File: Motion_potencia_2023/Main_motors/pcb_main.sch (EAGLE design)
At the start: 22 parts, among them IC1 TEENSY_4.1, X5 5566-25569-2, X6 5566-25569-2, X7 5566-25569-2, X8 5566-25569-2

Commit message: main lista, sin revisión
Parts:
- removed 12V_VENT, 3.3_MD, 5V_TEENSY, MOUT5, MOUT6, MOUT7, MOUT8, X5, X6, X7, X8: 5566-25569-2, molex_arreglado_2:5566-25569-2
- added 12V_IN, VENT1, VENT2: (no value), pinhead:PINHD-1X2
- added 5_MD: 5566-25569-2, molex_arreglado_2:5566-25569-2
- added FUSEMD1, FUSEMD2: FUSEBLANK_5X20MM, fuse:FUSEBLANK_5X20MM
- added JP1, JP3, JP4: (no value), pinhead:PINHD-1X4
- added RGB1, RGB2: (no value), pinhead:PINHD-1X3
- added U$1, U$2, U$3, U$4: GX16_2_PINS, Robocol_Eagle_Libraries2:GX16_2_PINS
- JP2: device jumper:JP4Q -> pinhead:PINHD-1X4
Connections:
- removed net 3.3V: JP2.7
- removed net 3.3V_MD: 3.3_MD-2.S, MD_1.VIN, MD_2.VIN
- removed net 5V_TEENSY: 5V_TEENSY-2.S, IC1.VIN_(3.6_TO_5.5_VOLTS)
- removed net N$1: X7-2.S, X8-2.S
- removed net SCL_1: JP2.1
- removed net SCL_2: JP2.3
- removed net SDA_1: JP2.2
- removed net SDA_2: JP2.4
- new net 5V_MD: 5_MD-2.S, JP1.1, JP2.1, JP3.1, JP4.1, MD_1.VIN, MD_2.VIN, RGB1.1, RGB2.1
- new net A14: IC1.A14, JP4.2
- new net A15: IC1.A15, JP3.2
- new net A16: IC1.A16, JP2.2
- new net A17: IC1.A17, JP1.2
- new net D18: IC1.A4, JP2.4
- new net D19: IC1.A5, JP1.4
- new net D28: IC1.RX7, RGB1.2
- new net D29: IC1.TX7, RGB2.2
- new net D36: IC1.CS_2, JP4.4
- new net D37: IC1.CS_3, JP3.4
- new net FUSE20AMD1: 24V_IZQ-2.S, FUSEMD1.2
- new net FUSE20AMD2: 24V_DER-2.S, FUSEMD2.2
- net 12V_VENT: now also 12V_IN.2, VENT1.2, VENT2.2; no longer 12V_VENT-2.S, X5-2.S, X6-2.S
- net 24V_IN_MD: now also FUSEMD1.1, FUSEMD2.1; no longer 24V_DER-2.S, 24V_IZQ-2.S
- net GND: now also 12V_IN.1, 5_MD-1.S, JP1.3, JP2.3, JP3.3, JP4.3, RGB1.3, RGB2.3, VENT1.1, VENT2.1; no longer 12V_VENT-1.S, 3.3_MD-1.S, 5V_TEENSY-1.S, JP2.8, X5-1.S, X6-1.S, X7-1.S, X8-1.S
- net N$10: now also MOUT3-2.S, U$3.1; no longer MOUT4-2.S, MOUT8-2.S
- net N$3: now also U$1.3; no longer MOUT5-1.S
- net N$4: now also MOUT2-1.S, U$2.3; no longer MOUT1-2.S, MOUT5-2.S
- net N$5: now also MOUT2-2.S, U$2.1; no longer MOUT2-1.S, MOUT6-1.S
- net N$6: now also MOUT1-2.S, U$1.1; no longer MOUT2-2.S, MOUT6-2.S
- net N$7: now also MOUT4-1.S, U$4.3; no longer MOUT3-1.S, MOUT7-1.S
- net N$8: now also MOUT4-2.S, U$4.1; no longer MOUT3-2.S, MOUT7-2.S
- net N$9: now also MOUT3-1.S, U$3.3; no longer MOUT4-1.S, MOUT8-1.S
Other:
- moved on the sheet: 24V_DER-1, 24V_DER-2, 24V_IZQ-1, 24V_IZQ-2, IC1, MD_1, MD_2, MOUT1-1, MOUT1-2, MOUT2-1, MOUT2-2, MOUT3-1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

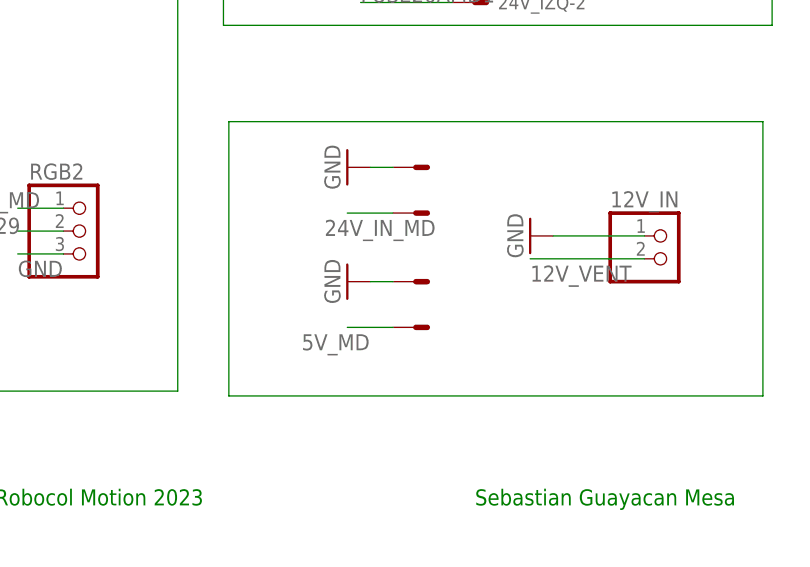
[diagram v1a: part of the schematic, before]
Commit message: main, power
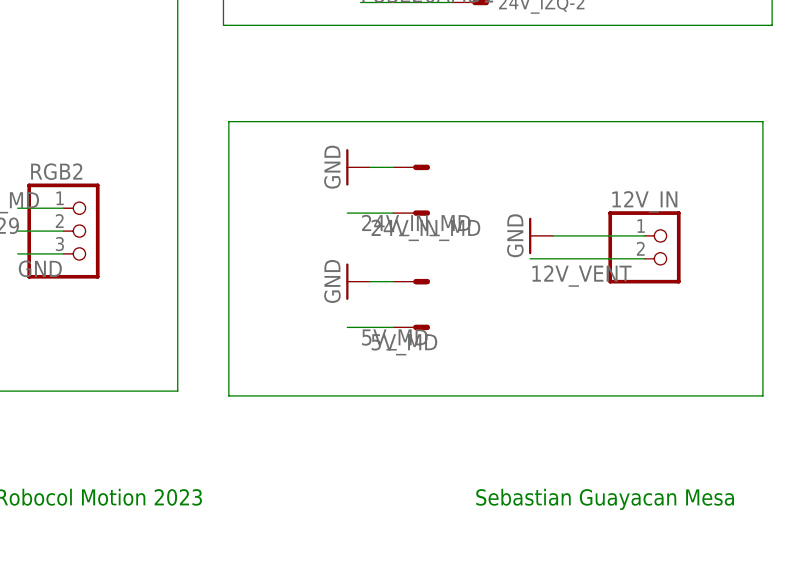
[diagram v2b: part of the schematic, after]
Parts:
- renumbered U$1 to M1, U$2 to M2, U$3 to M3, U$4 to M4
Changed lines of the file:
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@@
 <setting verticaltext="up"/>
 </settings>
-<grid distance="1" unitdist="mil" unit="mil" style="lines" multiple="1" display="no" altdistance="0.01" altunitdist="inch" altunit="inch"/>
+<grid distance="0.1" unitdist="inch" unit="inch" style="lines" multiple="1" display="no" altdistance="0.01" altunitdist="inch" altunit="inch"/>
 <layers>
 <layer number="1" name="Top" color="4" fill="1" visible="no" active="no"/>
@@
 <part name="GND5" library="supply1" library_urn="urn:adsk.eagle:library:371" deviceset="GND" device=""/>
 <part name="12V_IN" library="pinhead" library_urn="urn:adsk.eagle:library:325" deviceset="PINHD-1X2" device="" package3d_urn="urn:adsk.eagle:package:22435/2"/>
-<part name="U$1" library="Robocol_Eagle_Libraries2" deviceset="GX16_2_PINS" device=""/>
-<part name="U$2" library="Robocol_Eagle_Libraries2" deviceset="GX16_2_PINS" device=""/>
-<part name="U$3" library="Robocol_Eagle_Libraries2" deviceset="GX16_2_PINS" device=""/>
-<part name="U$4" library="Robocol_Eagle_Libraries2" deviceset="GX16_2_PINS" device=""/>
+<part name="M1" library="Robocol_Eagle_Libraries2" deviceset="GX16_2_PINS" device=""/>
+<part name="M2" library="Robocol_Eagle_Libraries2" deviceset="GX16_2_PINS" device=""/>
+<part name="M3" library="Robocol_Eagle_Libraries2" deviceset="GX16_2_PINS" device=""/>
+<part name="M4" library="Robocol_Eagle_Libraries2" deviceset="GX16_2_PINS" device=""/>
 <part name="FUSEMD1" library="fuse" library_urn="urn:adsk.eagle:library:233" deviceset="FUSE" device="BLANK_5X20MM" package3d_urn="urn:adsk.eagle:package:14079/1"/>
 <part name="FUSEMD2" library="fuse" library_urn="urn:adsk.eagle:library:233" deviceset="FUSE" device="BLANK_5X20MM" package3d_urn="urn:adsk.eagle:package:14079/1"/>
@@
 <attribute name="VALUE" x="233.47" y="42.64" size="1.778" layer="96"/>
 </instance>
-<instance part="U$1" gate="G$1" x="209.55" y="102.87" smashed="yes" rot="MR0"/>
-<instance part="U$2" gate="G$1" x="237.49" y="102.87" smashed="yes" rot="MR0"/>
-<instance part="U$3" gate="G$1" x="209.55" y="160.02" smashed="yes" rot="MR0"/>
-<instance part="U$4" gate="G$1" x="237.49" y="160.02" smashed="yes" rot="MR0"/>
+<instance part="M1" gate="G$1" x="209.55" y="102.87" smashed="yes" rot="MR0"/>
+<instance part="M2" gate="G$1" x="237.49" y="102.87" smashed="yes" rot="MR0"/>
+<instance part="M3" gate="G$1" x="209.55" y="160.02" smashed="yes" rot="MR0"/>
+<instance part="M4" gate="G$1" x="237.49" y="160.02" smashed="yes" rot="MR0"/>
 <instance part="FUSEMD1" gate="G$1" x="67.7418" y="19.1516" smashed="yes">
 <attribute name="NAME" x="63.9318" y="20.5486" size="1.778" layer="95"/>
@@
 <pinref part="24V_MD" gate="-2" pin="S"/>
 <wire x1="204.26" y1="52.8" x2="209.34" y2="52.8" width="0.1524" layer="91"/>
-<label x="201.72" y="50.26" size="1.778" layer="95"/>
+<label x="206.8" y="50.26" size="1.778" layer="95"/>
+<label x="205.74" y="50.8" size="1.778" layer="95"/>
 </segment>
 <segment>
@@
 <pinref part="5_MD" gate="-2" pin="S"/>
 <wire x1="209.34" y1="40.1" x2="204.26" y2="40.1" width="0.1524" layer="91"/>
-<label x="199.18" y="37.56" size="1.778" layer="95"/>
+<label x="206.8" y="37.56" size="1.778" layer="95"/>
+<label x="205.74" y="38.1" size="1.778" layer="95"/>
 </segment>
 <segment>
@@
 <net name="N$3" class="0">
 <segment>
-<pinref part="U$1" gate="G$1" pin="3"/>
+<pinref part="M1" gate="G$1" pin="3"/>
 <wire x1="198.12" y1="99.06" x2="198.12" y2="91.44" width="0.1524" layer="91"/>
 <pinref part="MOUT1" gate="-1" pin="S"/>
@@
 <segment>
 <pinref part="MOUT2" gate="-1" pin="S"/>
-<pinref part="U$2" gate="G$1" pin="3"/>
+<pinref part="M2" gate="G$1" pin="3"/>
 <wire x1="231.14" y1="91.44" x2="226.06" y2="91.44" width="0.1524" layer="91"/>
 <wire x1="226.06" y1="91.44" x2="226.06" y2="99.06" width="0.1524" layer="91"/>
@@
 <net name="N$5" class="0">
 <segment>
-<pinref part="U$2" gate="G$1" pin="1"/>
+<pinref part="M2" gate="G$1" pin="1"/>
 <wire x1="226.06" y1="106.68" x2="224.79" y2="106.68" width="0.1524" layer="91"/>
 <wire x1="224.79" y1="106.68" x2="224.79" y2="86.36" width="0.1524" layer="91"/>
@@
 <net name="N$6" class="0">
 <segment>
-<pinref part="U$1" gate="G$1" pin="1"/>
+<pinref part="M1" gate="G$1" pin="1"/>
 <wire x1="198.12" y1="106.68" x2="196.85" y2="105.41" width="0.1524" layer="91"/>
 <pinref part="MOUT1" gate="-2" pin="S"/>
@@
 <pinref part="MOUT4" gate="-1" pin="S"/>
 <wire x1="231.14" y1="149.86" x2="226.06" y2="149.86" width="0.1524" layer="91"/>
-<pinref part="U$4" gate="G$1" pin="3"/>
+<pinref part="M4" gate="G$1" pin="3"/>
 <wire x1="226.06" y1="149.86" x2="226.06" y2="156.21" width="0.1524" layer="91"/>
 </segment>
@@
 <wire x1="231.14" y1="144.78" x2="224.79" y2="144.78" width="0.1524" layer="91"/>
 <wire x1="224.79" y1="144.78" x2="224.79" y2="163.83" width="0.1524" layer="91"/>
-<pinref part="U$4" gate="G$1" pin="1"/>
+<pinref part="M4" gate="G$1" pin="1"/>
 <wire x1="224.79" y1="163.83" x2="226.06" y2="163.83" width="0.1524" layer="91"/>
 </segment>
@@
 <pinref part="MOUT3" gate="-1" pin="S"/>
 <wire x1="203.2" y1="148.59" x2="198.12" y2="148.59" width="0.1524" layer="91"/>
-<pinref part="U$3" gate="G$1" pin="3"/>
+<pinref part="M3" gate="G$1" pin="3"/>
 <wire x1="198.12" y1="148.59" x2="198.12" y2="156.21" width="0.1524" layer="91"/>
 </segment>
@@
 <net name="N$10" class="0">
 <segment>
-<pinref part="U$3" gate="G$1" pin="1"/>
+<pinref part="M3" gate="G$1" pin="1"/>
 <wire x1="198.12" y1="163.83" x2="196.85" y2="163.83" width="0.1524" layer="91"/>
 <pinref part="MOUT3" gate="-2" pin="S"/>
